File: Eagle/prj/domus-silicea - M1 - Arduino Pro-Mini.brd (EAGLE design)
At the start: 50.5 x 20.4 mm, 5 parts, among them M1 ARDUINO-PRO-MINI-3.3V

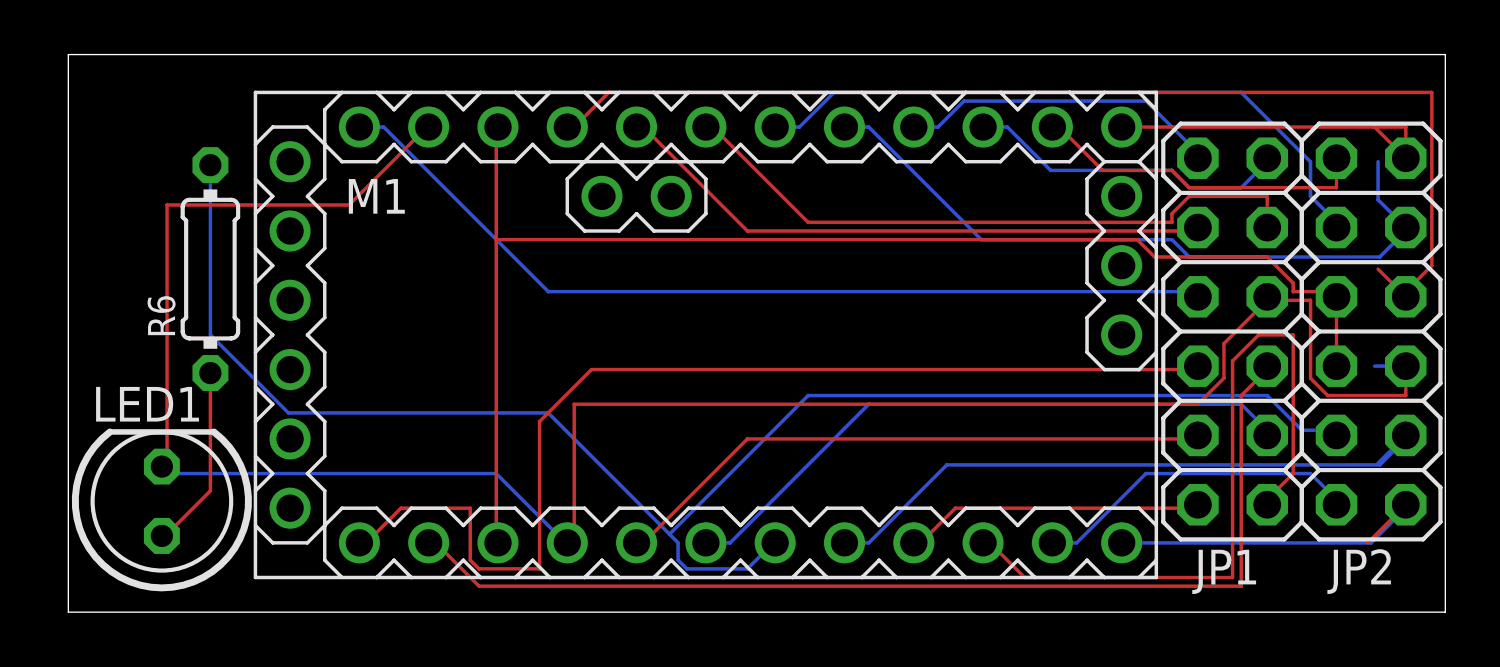
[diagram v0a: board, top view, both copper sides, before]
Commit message: EASYIOT_OLED
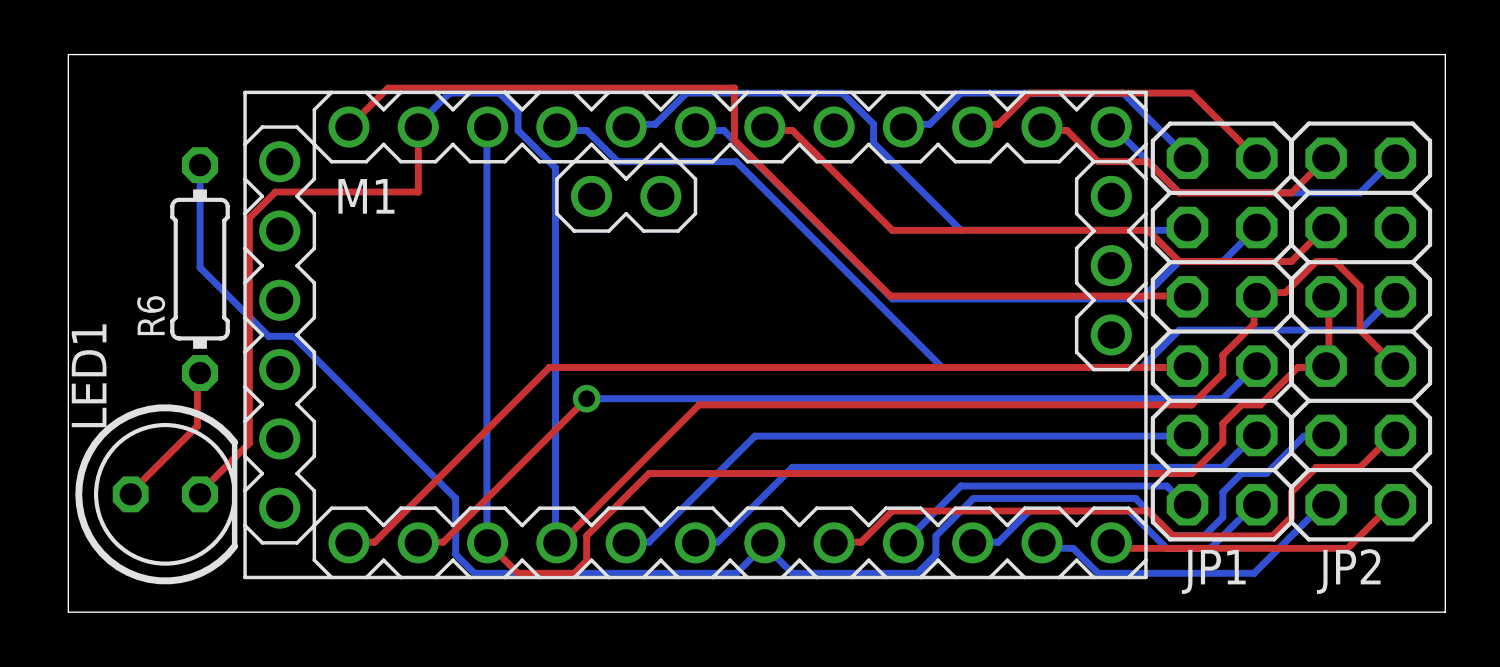
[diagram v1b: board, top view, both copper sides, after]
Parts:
- moved JP1 0.38 mm to (88.5, 10.9)
- moved JP2 0.38 mm to (93.6, 10.9)
- moved M1 0.38 mm to (69.2, 10.8)
- moved R6 0.38 mm to (51.1, 13.2)
- moved LED1 0.28 mm to (49.8, 4.95), turned to 0 degrees
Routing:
- net A0: track 25.9 -> 0.00 mm
- net D7: track 26.8 -> 12.3 mm
- net D1/TX: track 39.6 -> 33.4 mm
- net VCC: track 41.5 -> 35.4 mm
- net D0/RX: track 38.9 -> 33.4 mm, vias 0 -> 1
- net RST: track 49.9 -> 53.1 mm
- net D4: track 58.5 -> 56.0 mm
- net RAW: track 33.4 -> 35.6 mm
- net D9: track 13.0 -> 11.2 mm
- net A3: track 22.3 -> 23.6 mm
- net D10: track 13.2 -> 11.9 mm
- net N$6: track 6.76 -> 5.51 mm
- net D3: track 23.3 -> 22.2 mm
- net GND: track 80.1 -> 79.2 mm
- net A1: track 24.0 -> 23.1 mm
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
